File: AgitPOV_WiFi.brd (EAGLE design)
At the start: 41.5 x 67.6 mm, 42 parts

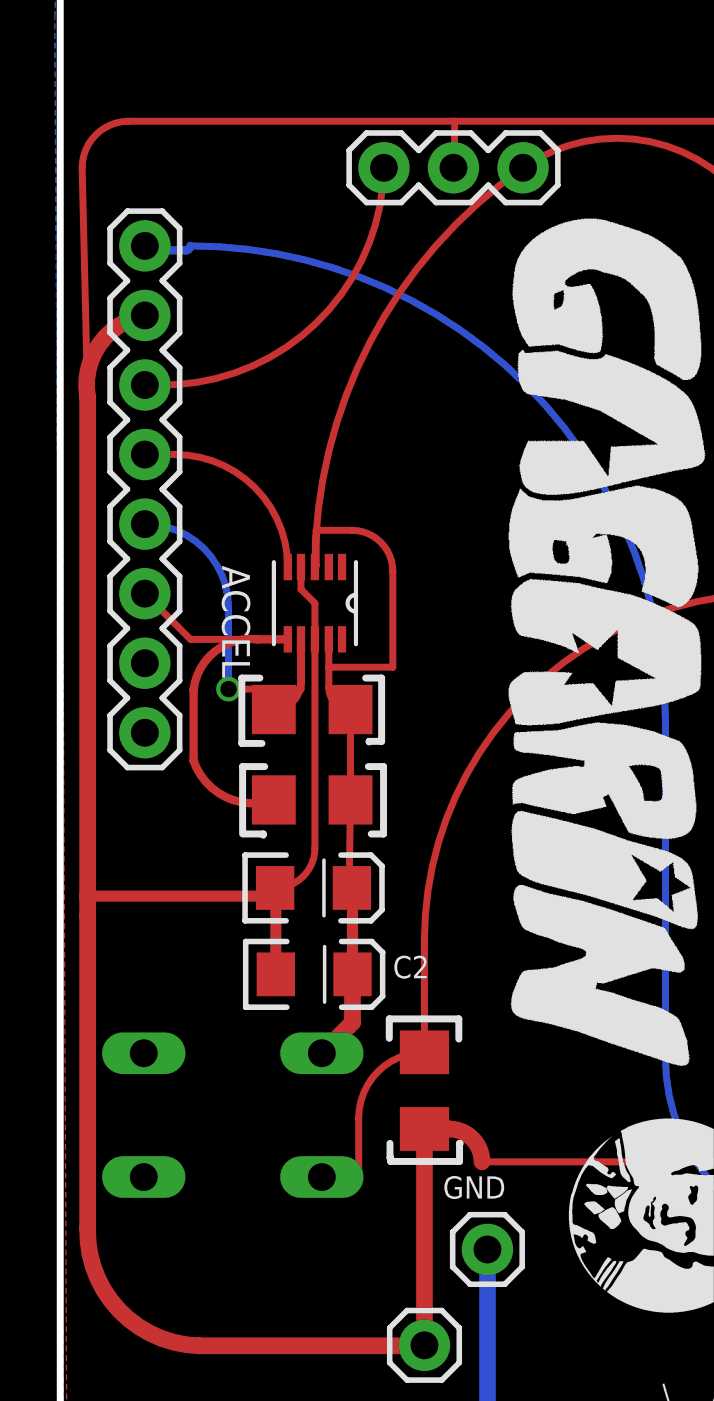
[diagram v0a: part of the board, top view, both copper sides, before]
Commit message: proper ACCEL integration
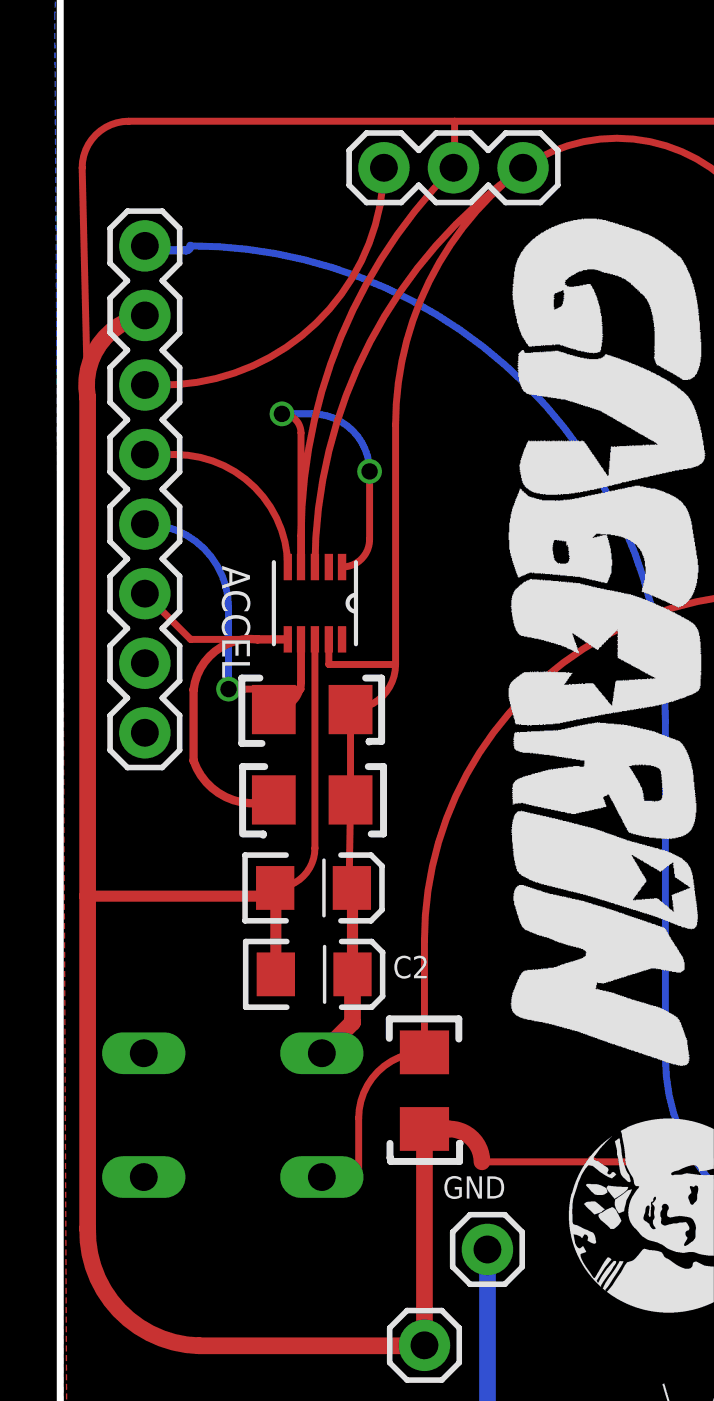
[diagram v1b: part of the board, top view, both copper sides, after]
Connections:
- net GND: now also ACCEL.1
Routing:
- net GND: track 313.7 -> 340.4 mm, vias 0 -> 2
- net +3.3V: track 52.5 -> 63.9 mm
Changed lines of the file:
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@@
 <contactref element="ACCEL" pad="8"/>
 <contactref element="JP-GND" pad="1"/>
-<wire x1="9.14608125" y1="45.5577625" x2="9.14608125" y2="44.7449625" width="0.254" layer="1"/>
-<wire x1="9.14608125" y1="44.7449625" x2="9.65408125" y2="44.2369625" width="0.254" layer="1"/>
-<wire x1="9.65408125" y1="44.2369625" x2="9.65408125" y2="42.9161625" width="0.254" layer="1"/>
 <wire x1="1.35408125" y1="51.7549625" x2="1.35408125" y2="33.5387625" width="0.6096" layer="1"/>
-<wire x1="1.35408125" y1="33.5387625" x2="1.35408125" y2="32.8026" width="0.6096" layer="1"/>
-<wire x1="1.35408125" y1="32.8026" x2="1.35408125" y2="21.40111875" width="0.6096" layer="1"/>
+<wire x1="1.35408125" y1="33.5387625" x2="1.35408125" y2="21.40111875" width="0.6096" layer="1"/>
 <wire x1="8.20328125" y1="33.8387625" x2="8.50328125" y2="33.5387625" width="0.254" layer="1" curve="-90"/>
 <wire x1="33.35408125" y1="61.7369625" x2="33.25408125" y2="61.8369625" width="0.254" layer="1" curve="90"/>
@@
 <wire x1="1.35408125" y1="21.40111875" x2="5.4356" y2="17.1196" width="0.6096" layer="1" curve="90"/>
 <wire x1="3.44408125" y1="54.7449625" x2="1.35408125" y2="51.7549625" width="0.6096" layer="1" curve="90"/>
+<wire x1="9.14608125" y1="45.5577625" x2="9.15" y2="46.7" width="0.254" layer="1"/>
+<wire x1="9.15" y1="46.7" x2="14.71408125" y2="60.1369625" width="0.254" layer="1" curve="-44.594558"/>
+<contactref element="ACCEL" pad="1"/>
+<wire x1="39.05408125" y1="56.5369625" x2="35.05408125" y2="56.5369625" width="0" layer="19" extent="1-16"/>
+<wire x1="10.64468125" y1="45.5577625" x2="11.65" y2="46.56308125" width="0.254" layer="1" curve="90"/>
+<wire x1="11.65" y1="46.56308125" x2="11.65" y2="49.05" width="0.254" layer="1"/>
+<via x="11.65" y="49.05" extent="1-16" drill="0.6" shape="square"/>
+<wire x1="11.65" y1="49.05" x2="9.55" y2="51.15" width="0.254" layer="16" curve="90"/>
+<wire x1="9.55" y1="51.15" x2="8.45" y2="51.15" width="0.254" layer="16"/>
+<via x="8.45" y="51.15" extent="1-16" drill="0.6" shape="square"/>
+<wire x1="8.45" y1="51.15" x2="9.14608125" y2="50.45391875" width="0.254" layer="1" curve="-90"/>
+<wire x1="9.14608125" y1="50.45391875" x2="9.14608125" y2="45.5577625" width="0.254" layer="1"/>
 </signal>
 <signal name="+3.3V">
@@
 <wire x1="10.90328125" y1="33.9387625" x2="10.95408125" y2="37.0529625" width="0.254" layer="1"/>
 <wire x1="10.95408125" y1="37.0529625" x2="10.95408125" y2="40.3529625" width="0.254" layer="1"/>
-<wire x1="10.95408125" y1="40.3529625" x2="10.16208125" y2="41.1449625" width="0.254" layer="1" curve="-90"/>
-<wire x1="10.16208125" y1="41.1449625" x2="10.16208125" y2="41.9" width="0.254" layer="1"/>
 <contactref element="PUSHBUTTON" pad="1"/>
-<wire x1="10.16208125" y1="41.9" x2="10.16208125" y2="42.9161625" width="0.254" layer="1"/>
 <wire x1="9.65408125" y1="45.5577625" x2="17.25408125" y2="60.1369625" width="0.254" layer="1" curve="-55.065212"/>
 <wire x1="17.25408125" y1="60.1369625" x2="26.30408125" y2="57.2849625" width="0.254" layer="1" curve="-104.852826"/>
@@
 <wire x1="11.0266" y1="30.6832" x2="11.0266" y2="28.92291875" width="0.6096" layer="1"/>
 <wire x1="11.0266" y1="28.92291875" x2="9.90671875" y2="27.8030375" width="0.6096" layer="1"/>
-<wire x1="9.65408125" y1="45.5577625" x2="9.7" y2="45.60368125" width="0.254" layer="1" curve="90"/>
-<wire x1="9.7" y1="45.60368125" x2="9.7" y2="46.9" width="0.254" layer="1"/>
-<wire x1="9.7" y1="46.9" x2="11" y2="46.9" width="0.254" layer="1"/>
-<wire x1="11" y1="46.9" x2="12.5" y2="45.4" width="0.254" layer="1" curve="-90"/>
-<wire x1="12.5" y1="45.4" x2="12.5" y2="41.9" width="0.254" layer="1"/>
-<wire x1="12.5" y1="41.9" x2="10.16208125" y2="41.9" width="0.254" layer="1"/>
+<wire x1="10.95408125" y1="40.3529625" x2="12.6" y2="41.99888125" width="0.254" layer="1" curve="90"/>
+<wire x1="12.6" y1="41.99888125" x2="12.6" y2="50.75" width="0.254" layer="1"/>
+<wire x1="12.6" y1="50.75" x2="17.25408125" y2="60.1369625" width="0.254" layer="1" curve="-52.744681"/>
+<wire x1="12.6" y1="41.99888125" x2="10.16208125" y2="41.99888125" width="0.254" layer="1"/>
+<wire x1="10.16208125" y1="41.99888125" x2="10.16208125" y2="42.9161625" width="0.254" layer="1"/>
 </signal>
 <signal name="N$6">
